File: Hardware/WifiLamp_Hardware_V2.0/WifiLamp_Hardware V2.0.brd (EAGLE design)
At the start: 100 x 80 mm, 24 parts, among them CN1 MKDSN1,5/2-5,08, CN3 MKDSN1,5/2-5,08, CN4 MKDSN1,5/2-5,08, T1 BTA12, U1 LM1117, U2 MOC3041M

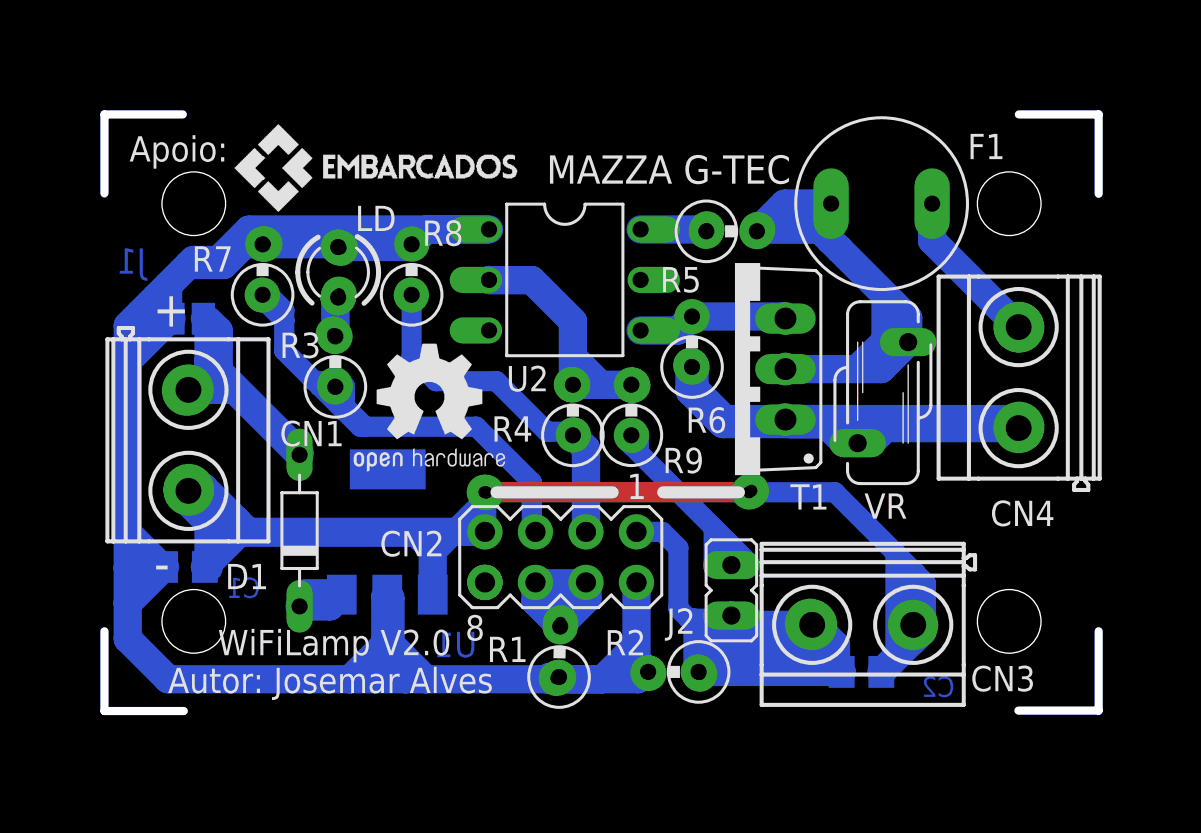
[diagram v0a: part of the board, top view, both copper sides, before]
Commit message: Inclusão dos gerbers e BOM do hardware V2
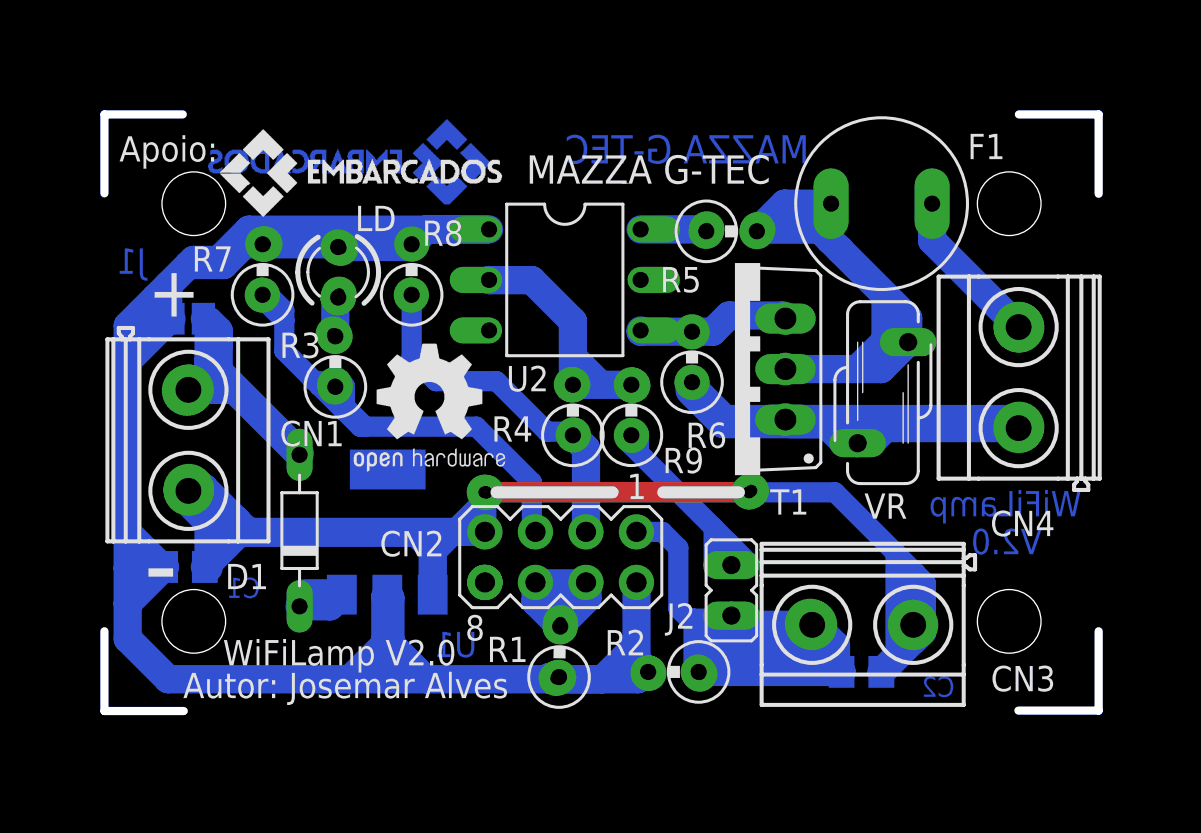
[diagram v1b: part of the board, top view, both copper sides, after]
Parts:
- moved R6 0.76 mm to (55.6, 37.8)
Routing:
- net N$72: track 23.4 -> 22.6 mm

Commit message: Inclusao do firmware e app
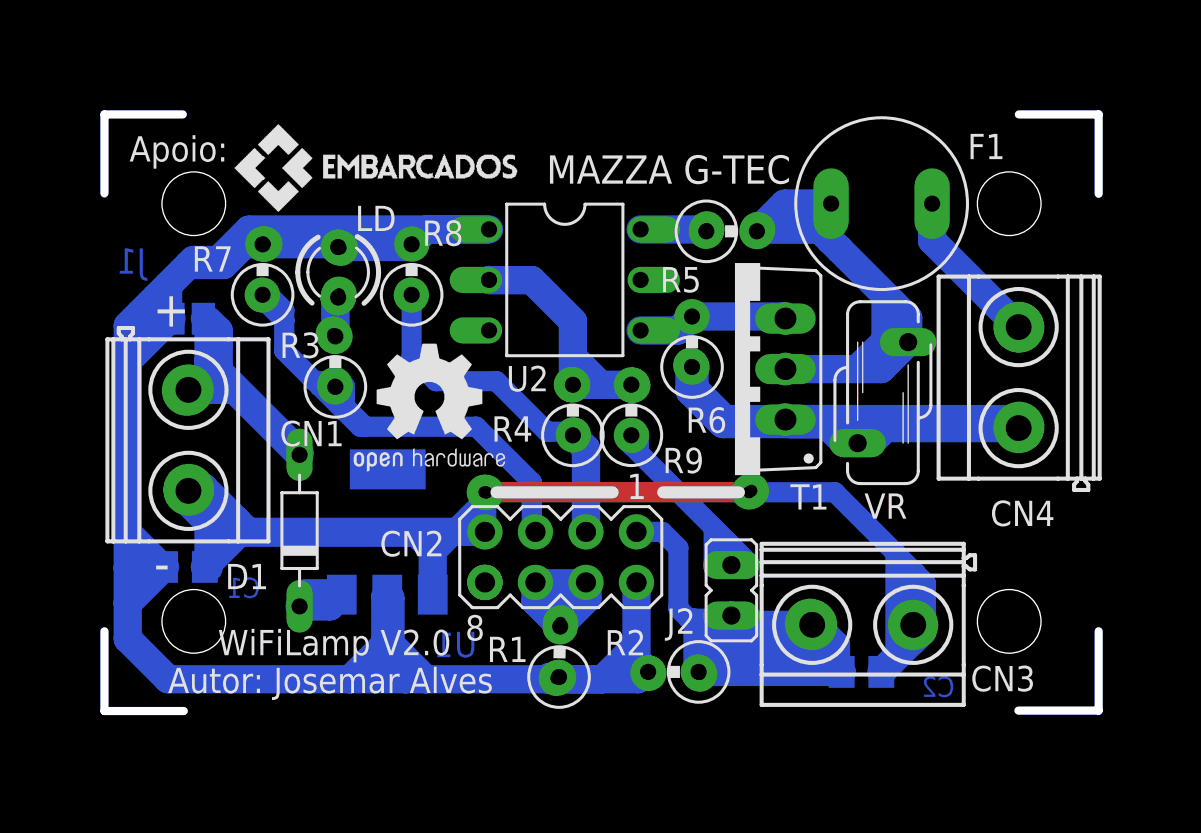
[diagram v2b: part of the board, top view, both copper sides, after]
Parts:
- moved R6 0.76 mm to (55.6, 38.6)
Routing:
- net N$72: track 22.6 -> 23.4 mm
